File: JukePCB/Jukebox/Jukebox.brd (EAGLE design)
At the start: 133.5 x 197 mm, 31 parts, among them CN1 1X4-BIG

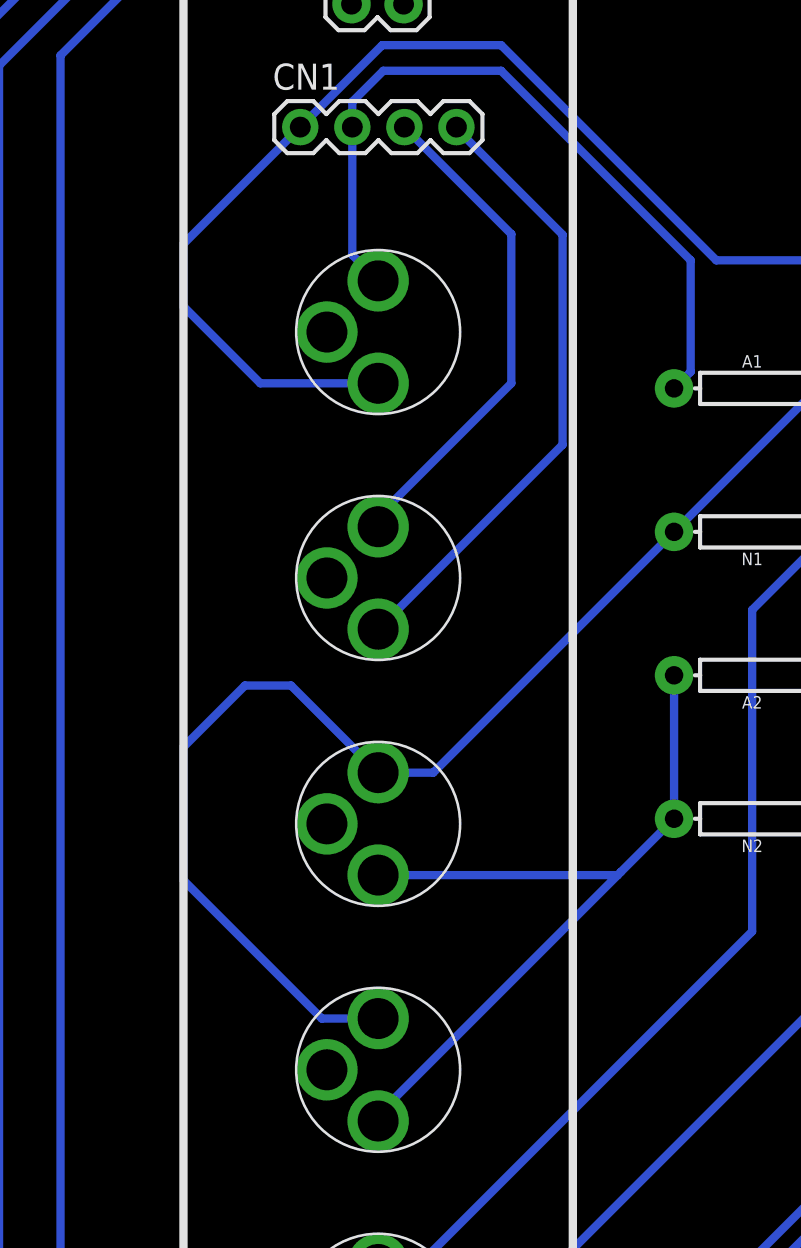
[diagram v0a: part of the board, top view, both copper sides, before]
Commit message: Huge Sound Update, almost final
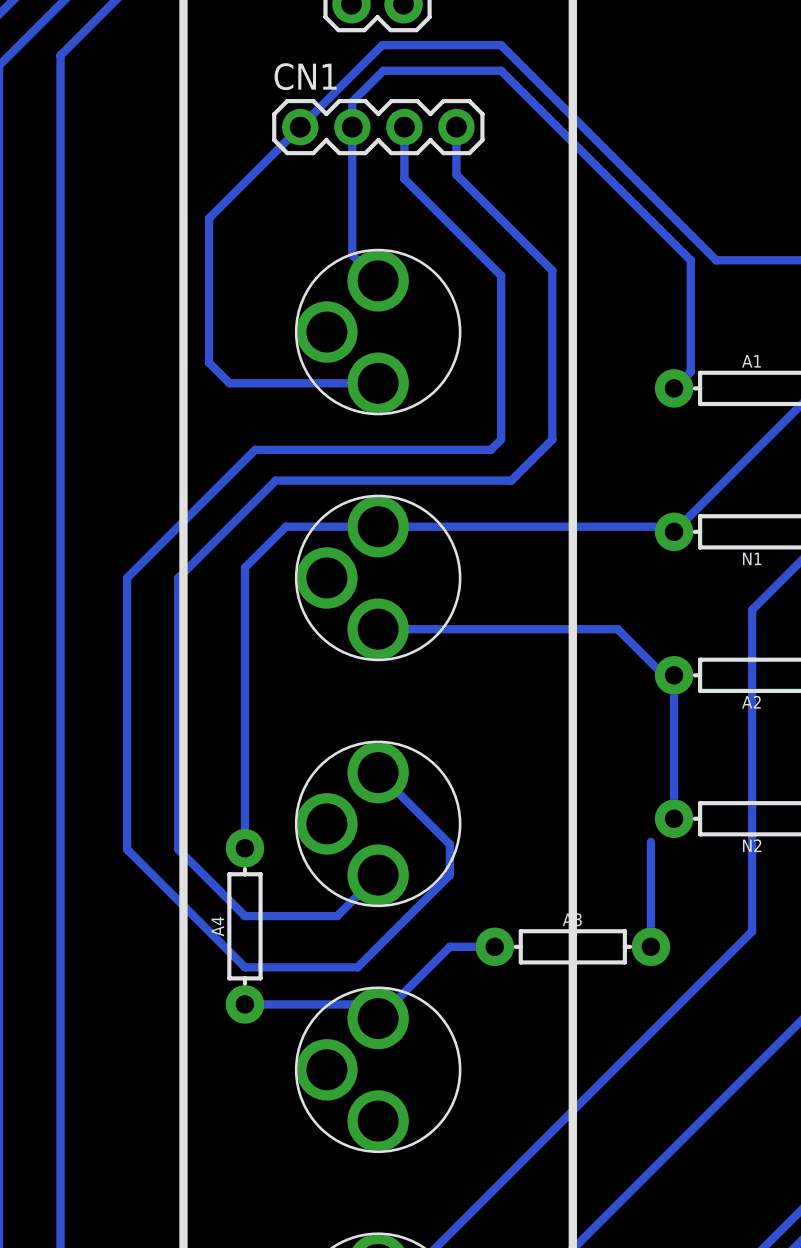
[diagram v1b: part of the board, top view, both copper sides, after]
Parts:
- added A3, A4: 1k, SparkFun-Resistors:AXIAL-0.3
- moved AUXOUT 12.0 mm to (-34.5, 26.0)
- moved TOAMP 12.0 mm to (-34.5, 14.0)
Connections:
- new net N$38: A3.P$1, A4.P$1, TOLIGHT.2
- net GND: now also TOLIGHT.3
- net N$23: now also A3.P$2; no longer TOLIGHT.3
- net N$24: now also A4.P$2; no longer TOLIGHT.2
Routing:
- net N$13: track 24.4 -> 77.9 mm
- net N$14: track 30.4 -> 63.4 mm
- net N$24: track 61.1 -> 46.1 mm
- net N$38: track 0.00 -> 13.9 mm
- net N$23: track 39.4 -> 27.7 mm
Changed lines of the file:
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@@
 <element name="U$13" library="Jukebox" package="JUKEBUTTON" value="JUKEBUTTON" x="43.25" y="-86" rot="R90"/>
 <element name="U$14" library="Jukebox" package="JUKESWITCH" value="JUKESWITCH" x="27.25" y="-86"/>
-<element name="TOAMP" library="Jukebox" package="JUKEHEADPHONE" value="JUKEHEADPHONE" x="-34.5" y="26" rot="R90"/>
-<element name="AUXOUT" library="Jukebox" package="JUKEHEADPHONE" value="JUKEHEADPHONE" x="-34.5" y="14" rot="R90"/>
+<element name="TOAMP" library="Jukebox" package="JUKEHEADPHONE" value="JUKEHEADPHONE" x="-34.5" y="14" rot="R90"/>
+<element name="AUXOUT" library="Jukebox" package="JUKEHEADPHONE" value="JUKEHEADPHONE" x="-34.5" y="26" rot="R90"/>
 <element name="U$17" library="Jukebox" package="8PINJUKE" value="8PINJUKE2" x="60.25" y="-72.25" rot="R270"/>
 <element name="TOLIGHT" library="Jukebox" package="JUKEHEADPHONE" value="JUKEHEADPHONE" x="-34.5" y="2" rot="R90"/>
@@
 <element name="CONTROL1" library="adafruit" package="1X04-BIG" value="1X4-BIG" x="-30.7" y="-26" rot="R180"/>
 <element name="CONTROL2" library="adafruit" package="1X04-BIG" value="1X4-BIG" x="-30.7" y="-29" rot="R180"/>
+<element name="A3" library="SparkFun-Resistors" package="AXIAL-0.3" value="1k" x="-25" y="8">
+<attribute name="PROD_ID" value="RES-12183" x="-25" y="8" size="1.778" layer="27" display="off"/>
+</element>
+<element name="A4" library="SparkFun-Resistors" package="AXIAL-0.3" value="1k" x="-41" y="9" rot="R90">
+<attribute name="PROD_ID" value="RES-12183" x="-41" y="9" size="1.778" layer="27" rot="R90" display="off"/>
+</element>
 </elements>
 <signals>
@@
 <wire x1="-5.5" y1="28.19" x2="-12.44" y2="21.25" width="0.4064" layer="16"/>
 <wire x1="-38.3" y1="48" x2="-38.5" y2="48" width="0.4064" layer="16"/>
-<wire x1="-34.5" y1="35.5" x2="-40.25" y2="35.5" width="0.4064" layer="16"/>
-<wire x1="-40.25" y1="35.5" x2="-44" y2="39.25" width="0.4064" layer="16"/>
-<wire x1="-44" y1="39.25" x2="-44" y2="42.3" width="0.4064" layer="16"/>
-<wire x1="-44" y1="42.3" x2="-38.3" y2="48" width="0.4064" layer="16"/>
+<wire x1="-34.5" y1="35.5" x2="-41.75" y2="35.5" width="0.4064" layer="16"/>
+<wire x1="-41.75" y1="35.5" x2="-42.75" y2="36.5" width="0.4064" layer="16"/>
+<wire x1="-42.75" y1="36.5" x2="-42.75" y2="43.55" width="0.4064" layer="16"/>
+<wire x1="-42.75" y1="43.55" x2="-38.3" y2="48" width="0.4064" layer="16"/>
 </signal>
 <signal name="N$23">
@@
 <contactref element="N2" pad="P$2"/>
 <contactref element="AUXOUT" pad="3"/>
-<contactref element="TOLIGHT" pad="3"/>
-<wire x1="-20.06" y1="14.25" x2="-20.06" y2="21.25" width="0.4064" layer="16"/>
-<wire x1="-34.5" y1="-0.5" x2="-34.5" y2="-0.19" width="0.4064" layer="16"/>
-<wire x1="-34.5" y1="-0.19" x2="-22.81" y2="11.5" width="0.4064" layer="16"/>
-<wire x1="-22.655" y1="11.655" x2="-20.06" y2="14.25" width="0.4064" layer="16"/>
-<wire x1="-34.5" y1="11.5" x2="-22.81" y2="11.5" width="0.4064" layer="16"/>
-<wire x1="-22.81" y1="11.5" x2="-22.655" y2="11.655" width="0.4064" layer="16"/>
+<wire x1="-20.06" y1="14.25" x2="-20.06" y2="20.75" width="0.4064" layer="16"/>
+<contactref element="A3" pad="P$2"/>
+<wire x1="-20.06" y1="20.75" x2="-20.06" y2="21.25" width="0.4064" layer="16"/>
+<wire x1="-21.19" y1="8" x2="-21.19" y2="13.12" width="0.4064" layer="16"/>
+<wire x1="-34.5" y1="23.5" x2="-22.81" y2="23.5" width="0.4064" layer="16"/>
+<wire x1="-22.81" y1="23.5" x2="-20.06" y2="20.75" width="0.4064" layer="16"/>
+<wire x1="-20.06" y1="14.25" x2="-21.19" y2="13.12" width="0" layer="19" extent="16-16"/>
 </signal>
 <signal name="N$24">
@@
 <contactref element="A1" pad="P$2"/>
 <contactref element="AUXOUT" pad="2"/>
-<contactref element="TOLIGHT" pad="2"/>
 <wire x1="-12.44" y1="35.25" x2="-13.06" y2="35.25" width="0.4064" layer="16"/>
 <wire x1="-13.06" y1="35.25" x2="-20.06" y2="28.25" width="0.4064" layer="16"/>
-<wire x1="-34.5" y1="16.5" x2="-31.81" y2="16.5" width="0.4064" layer="16"/>
-<wire x1="-31.81" y1="16.5" x2="-20.06" y2="28.25" width="0.4064" layer="16"/>
-<wire x1="-34.5" y1="4.5" x2="-37.25" y2="4.5" width="0.4064" layer="16"/>
-<wire x1="-37.25" y1="4.5" x2="-44" y2="11.25" width="0.4064" layer="16"/>
-<wire x1="-44" y1="11.25" x2="-44" y2="17.75" width="0.4064" layer="16"/>
-<wire x1="-44" y1="17.75" x2="-41" y2="20.75" width="0.4064" layer="16"/>
-<wire x1="-41" y1="20.75" x2="-38.75" y2="20.75" width="0.4064" layer="16"/>
-<wire x1="-38.75" y1="20.75" x2="-34.5" y2="16.5" width="0.4064" layer="16"/>
+<contactref element="A4" pad="P$2"/>
+<wire x1="-34.5" y1="28.5" x2="-20.31" y2="28.5" width="0.4064" layer="16"/>
+<wire x1="-20.31" y1="28.5" x2="-20.06" y2="28.25" width="0.4064" layer="16"/>
+<wire x1="-41" y1="12.81" x2="-41" y2="26.5" width="0.4064" layer="16"/>
+<wire x1="-41" y1="26.5" x2="-39" y2="28.5" width="0.4064" layer="16"/>
+<wire x1="-39" y1="28.5" x2="-34.5" y2="28.5" width="0.4064" layer="16"/>
 </signal>
 <signal name="N$27">
@@
 </polygon>
 <contactref element="U$8" pad="12"/>
+<contactref element="TOLIGHT" pad="3"/>
 </signal>
 <signal name="N$22">
@@
 <contactref element="CN1" pad="3"/>
 <contactref element="TOAMP" pad="2"/>
-<wire x1="-34.5" y1="28.5" x2="-34.5" y2="29" width="0.4064" layer="16"/>
-<wire x1="-34.5" y1="29" x2="-28" y2="35.5" width="0.4064" layer="16"/>
-<wire x1="-28" y1="35.5" x2="-28" y2="42.78" width="0.4064" layer="16"/>
-<wire x1="-28" y1="42.78" x2="-33.22" y2="48" width="0.4064" layer="16"/>
+<wire x1="-33.22" y1="48" x2="-33.22" y2="45.47" width="0.4064" layer="16"/>
+<wire x1="-33.22" y1="45.47" x2="-28.5" y2="40.75" width="0.4064" layer="16"/>
+<wire x1="-28.5" y1="40.75" x2="-28.5" y2="32.75" width="0.4064" layer="16"/>
+<wire x1="-28.5" y1="32.75" x2="-29" y2="32.25" width="0.4064" layer="16"/>
+<wire x1="-29" y1="32.25" x2="-40.5" y2="32.25" width="0.4064" layer="16"/>
+<wire x1="-40.5" y1="32.25" x2="-46.75" y2="26" width="0.4064" layer="16"/>
+<wire x1="-46.75" y1="26" x2="-46.75" y2="12.75" width="0.4064" layer="16"/>
+<wire x1="-46.75" y1="12.75" x2="-41" y2="7" width="0.4064" layer="16"/>
+<wire x1="-41" y1="7" x2="-35.5" y2="7" width="0.4064" layer="16"/>
+<wire x1="-35.5" y1="7" x2="-31" y2="11.5" width="0.4064" layer="16"/>
+<wire x1="-31" y1="11.5" x2="-31" y2="13" width="0.4064" layer="16"/>
+<wire x1="-31" y1="13" x2="-34.5" y2="16.5" width="0.4064" layer="16"/>
 </signal>
 <signal name="N$14">
 <contactref element="TOAMP" pad="3"/>
 <contactref element="CN1" pad="4"/>
-<wire x1="-30.68" y1="48" x2="-30.68" y2="47.93" width="0.4064" layer="16"/>
-<wire x1="-30.68" y1="47.93" x2="-25.5" y2="42.75" width="0.4064" layer="16"/>
-<wire x1="-25.5" y1="42.75" x2="-25.5" y2="32.5" width="0.4064" layer="16"/>
-<wire x1="-25.5" y1="32.5" x2="-34.5" y2="23.5" width="0.4064" layer="16"/>
+<wire x1="-30.68" y1="48" x2="-30.68" y2="45.68" width="0.4064" layer="16"/>
+<wire x1="-30.68" y1="45.68" x2="-26" y2="41" width="0.4064" layer="16"/>
+<wire x1="-26" y1="41" x2="-26" y2="32.75" width="0.4064" layer="16"/>
+<wire x1="-26" y1="32.75" x2="-28" y2="30.75" width="0.4064" layer="16"/>
+<wire x1="-28" y1="30.75" x2="-39.5" y2="30.75" width="0.4064" layer="16"/>
+<wire x1="-39.5" y1="30.75" x2="-44.25" y2="26" width="0.4064" layer="16"/>
+<wire x1="-44.25" y1="26" x2="-44.25" y2="12.75" width="0.4064" layer="16"/>
+<wire x1="-44.25" y1="12.75" x2="-41" y2="9.5" width="0.4064" layer="16"/>
+<wire x1="-41" y1="9.5" x2="-36.5" y2="9.5" width="0.4064" layer="16"/>
+<wire x1="-36.5" y1="9.5" x2="-34.5" y2="11.5" width="0.4064" layer="16"/>
 </signal>
 <signal name="N$15">
@@
 </polygon>
 </signal>
+<signal name="N$38">
+<contactref element="TOLIGHT" pad="2"/>
+<contactref element="A4" pad="P$1"/>
+<wire x1="-41" y1="5.19" x2="-35.19" y2="5.19" width="0.4064" layer="16"/>
+<wire x1="-35.19" y1="5.19" x2="-34.5" y2="4.5" width="0.4064" layer="16"/>
+<contactref element="A3" pad="P$1"/>
+<wire x1="-28.81" y1="8" x2="-31" y2="8" width="0.4064" layer="16"/>
+<wire x1="-31" y1="8" x2="-34.5" y2="4.5" width="0.4064" layer="16"/>
+</signal>
 </signals>
